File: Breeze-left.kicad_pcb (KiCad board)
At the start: 2 copper layers, 210.6 x 114.9 mm, 103 parts, among them SW1 CHOCXHSPCB-1U, SW10 CHOCXHSPCB-1U, SW11 CHOCXHSPCB-1U, SW12 CHOCXHSPCB-1U, SW13 CHOCXHSPCB-1U, SW14 CHOCXHSPCB-1U, SW15 CHOCXHSPCB-1U, SW16 CHOCXHSPCB-1U, SW17 CHOCXHSPCB-1U, SW18 CHOCXHSPCB-1U, SW19 CHOCXHSPCB-1U, SW2 CHOCXHSPCB-1U, SW20 CHOCXHSPCB-1U, SW21 CHOCXHSPCB-1U, SW22 CHOCXHSPCB-1U, SW23 CHOCXHSPCB-1U, SW24 CHOCXHSPCB-1U, SW3 CHOCXHSPCB-1U, SW4 CHOCXHSPCB-1U, SW5 CHOCXHSPCB-1U, SW6 CHOCXHSPCB-1U, SW7 CHOCXHSPCB-1U, SW8 CHOCXHSPCB-1U, SW9 CHOCXHSPCB-1U

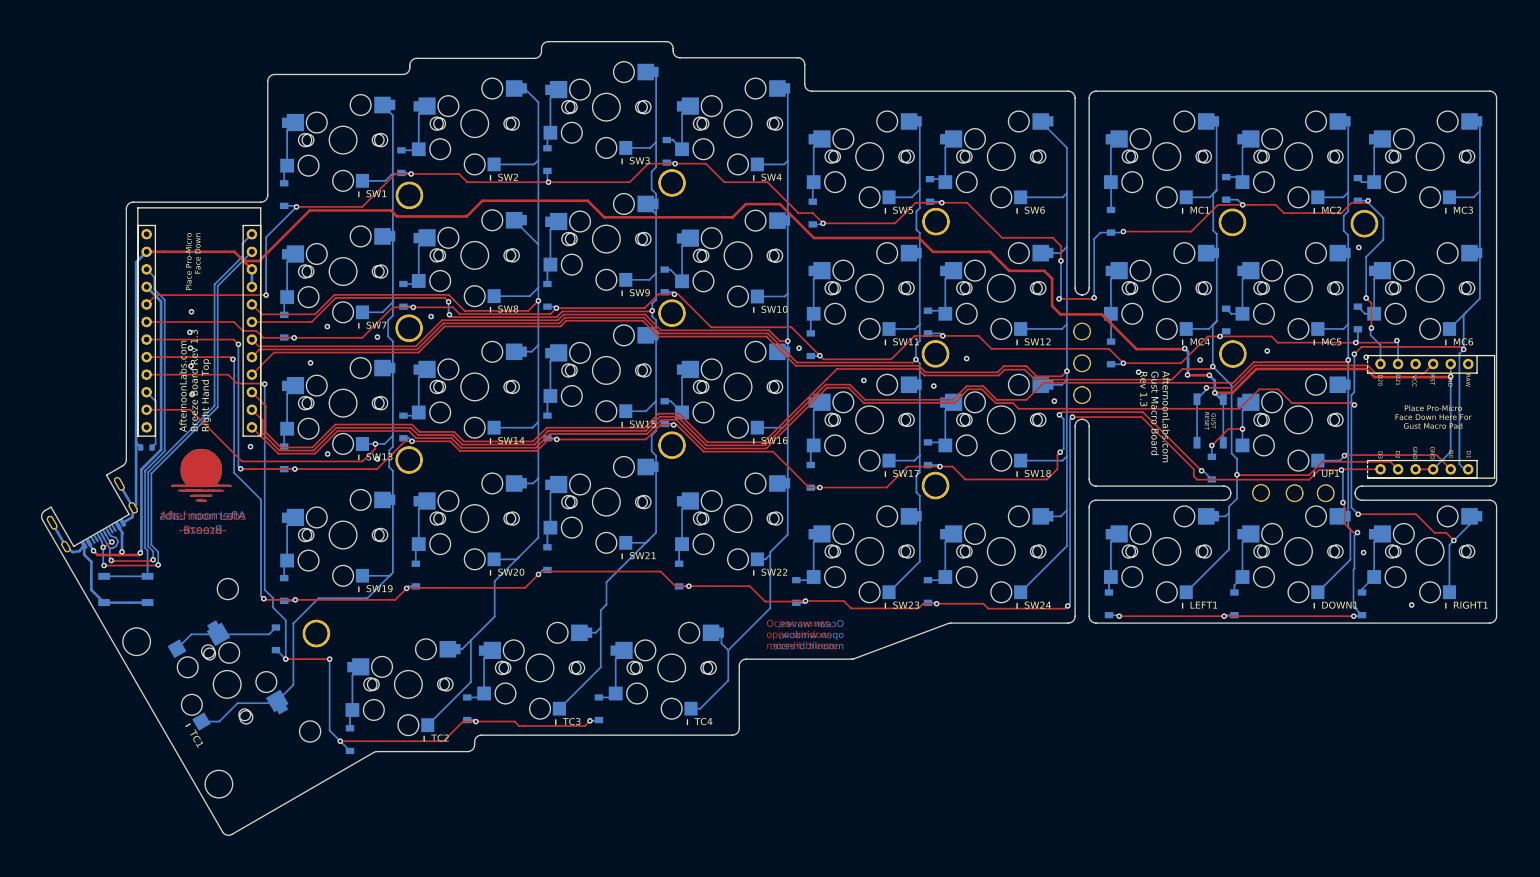
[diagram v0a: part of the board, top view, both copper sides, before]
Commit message: Route left hal
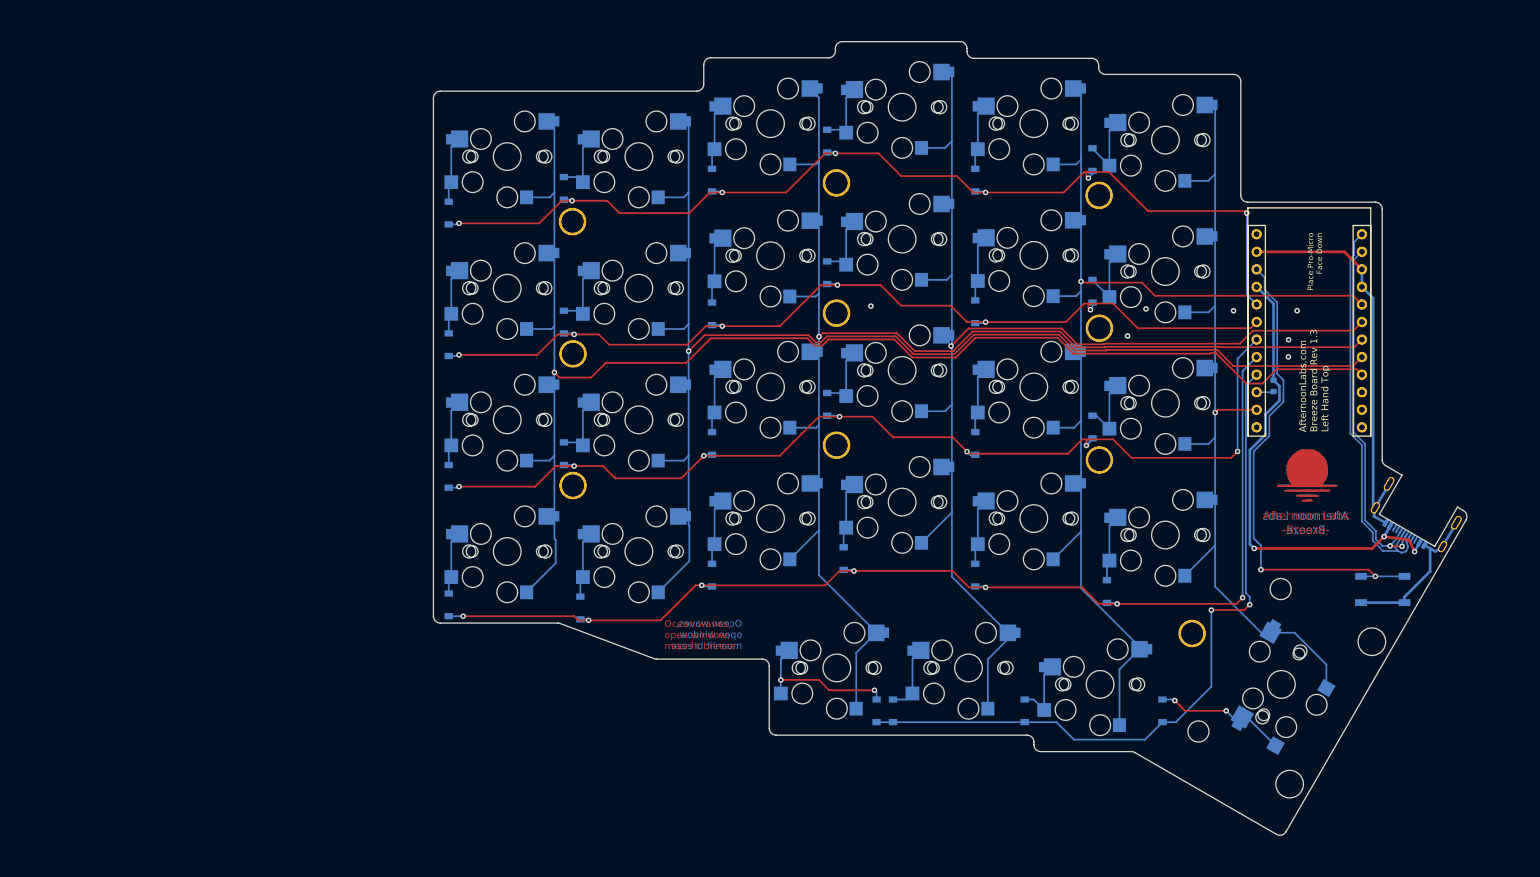
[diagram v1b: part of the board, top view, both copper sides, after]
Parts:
- removed DALF1, DAN1, DMC1, DMC2, DMC3, DMC4, DMC5, DMC6, DRT1, DUP1: DIODE, Breeze:SOD-123FL
- removed DOWN1, LEFT1, MC1, MC2, MC3, MC4, MC5, MC6, RIGHT1, UP1: CHOCXHSPCB-1U, Breeze:MX_Choc_Hotswap_1-Sided
- removed H1, H16, H17: M3-HOLE, Breeze:M3-HOLE
- removed H10, H11, H12, H13, H14, H15: 2M-HOLE, Breeze:M2-HOLE
- removed MCU-MACRO1: ProMicro-Partial, Breeze:PROMICRO-PARTIAL2
- removed RSW-MACRO1: SW-RST, Button_Switch_SMD:SW_SPST_TL3342
- H18, H19, H2, H3, H4, H5, H6, H7, H8, H9, LGO1, STABL1: moved to B.Cu
- moved USB1 195.6 mm to (303.6, 158.9), turned to 150 degrees
- moved RSW1 181.9 mm to (296.8, 173.2)
- moved R1 163.4 mm to (281.0, 143.8), turned to 90 degrees
- moved MCU-MAIN1 160.6 mm to (286.2, 135.8)
- moved LGO1 160.2 mm to (285.9, 156.7), turned to 180 degrees
- moved STABL1 152.6 mm to (282.1, 187.0), turned to -120 degrees
- moved TC1 152.6 mm to (282.1, 187.0), turned to 60 degrees
- moved DTC1 128.7 mm to (264.9, 190.8)
- moved H9 126.7 mm to (269.2, 179.6), turned to 180 degrees
- moved D19 119.1 mm to (256.9, 173.5)
- moved SW1 119.0 mm to (265.3, 108.2)
- moved SW13 119.0 mm to (265.3, 146.3)
- moved SW19 119.0 mm to (265.3, 165.4)
- moved SW7 119.0 mm to (265.3, 127.2)
- moved D1 117.1 mm to (254.8, 111.0)
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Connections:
- MCU-MAIN1 pad 10: COL6 -> unconnected-(MCU-MAIN1-D7(PE6)-Pad10)
- MCU-MAIN1 pad 11: COL7 -> unconnected-(MCU-MAIN1-D8(PB4)-Pad11)
- MCU-MAIN1 pad 12: COL8 -> unconnected-(MCU-MAIN1-D9(PB5)-Pad12)
- R1 pad 2: GND -> VCC
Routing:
- net COL8: track 304.6 -> 0.00 mm, vias 5 -> 0
- net COL7: track 278.3 -> 0.00 mm, vias 2 -> 0
- net COL6: track 268.0 -> 0.00 mm, vias 2 -> 0
- net GND: track 314.0 -> 81.6 mm, vias 29 -> 7
- net ROW3: track 317.6 -> 163.6 mm, vias 16 -> 7
- net ROW0: track 258.7 -> 149.0 mm, vias 15 -> 7
- net ROW1: track 212.4 -> 136.0 mm, vias 10 -> 6
- net ROW2: track 203.8 -> 150.3 mm, vias 11 -> 7
- net COL0: track 167.8 -> 120.7 mm
- net Net-(MCU-MACRO1-RST): track 43.7 -> 0.00 mm, vias 1 -> 0
- net COL1: track 183.6 -> 157.8 mm
- net COL5: track 231.4 -> 209.8 mm
- net ROW4: track 122.1 -> 103.8 mm, vias 6 -> 2
- net RST: track 53.1 -> 70.5 mm, vias 0 -> 2
- net VCC: track 53.8 -> 69.6 mm
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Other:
- board size 210.6 x 114.9 mm -> 149.6 x 114.9 mm
- board text added: "AfternoonLabs.com Breeze Board Rev 1.3 Left Hand Top"
- board text removed: "AfternoonLabs.com Breeze Board Rev 1.3 Right Hand Top"
- board text removed: "AfternoonLabs.com Gust Macro Board Rev 1.3"
- board text removed: "D0"
- board text removed: "D1"
- board text removed: "D2"
- board text removed: "D20"
- board text removed: "D21"
- board text removed: "D3"
- board text removed: "GND"
- board text removed: "GUST RESET"
- board text removed: "Place Pro-Micro Face Down Here For Gust Macro Pad"
- board text removed: "RAW"
- board text removed: "RST"
- board text removed: "VCC"
